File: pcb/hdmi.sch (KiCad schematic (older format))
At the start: 11 parts, among them U7 TPD12S016PWR, X5 HDMI_A

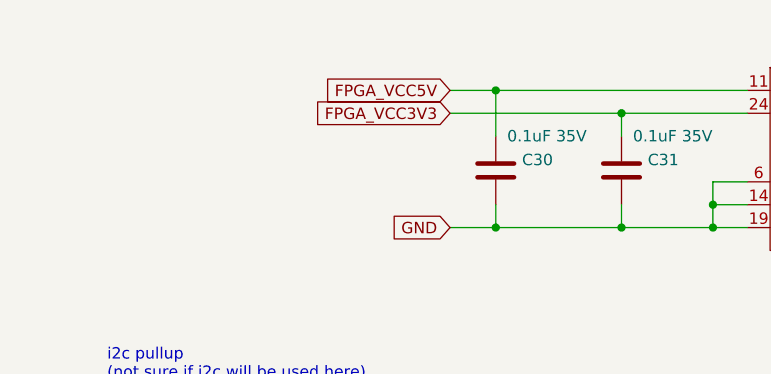
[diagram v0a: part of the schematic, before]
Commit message: Some more work done
I'm too lazy to think about commit messages in my pet project, really
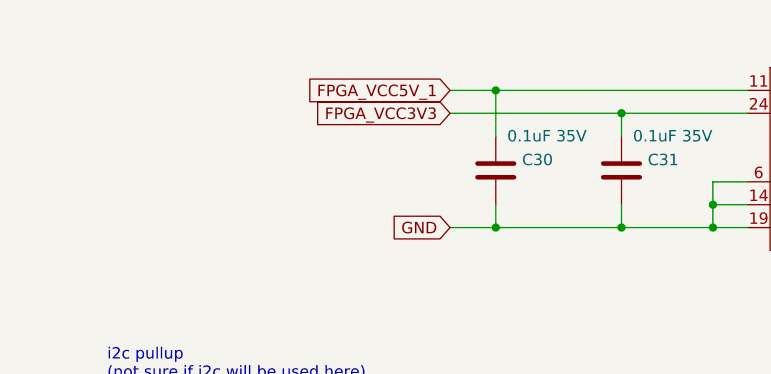
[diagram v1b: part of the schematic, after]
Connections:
- net FPGA_VCC5V renamed FPGA_VCC5V_1
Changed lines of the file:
@@
 $Descr A4 11693 8268
 encoding utf-8
-Sheet 12 11
+Sheet 11 11
 Title "Wishmaster 1200"
 Date ""
@@
 	6300 800  6300 1150
 Text GLabel 2700 800  0    50   Input ~ 0
-FPGA_VCC5V
+FPGA_VCC5V_1
 Text GLabel 2700 900  0    50   Input ~ 0
 FPGA_VCC3V3
